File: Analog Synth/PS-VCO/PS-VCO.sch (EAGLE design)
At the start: 44 parts, among them IC1 TL084D, Q1 BC847BS, Q2 2N3906, Q3 2N3904, Q4 2N3904, Q5 2N7000

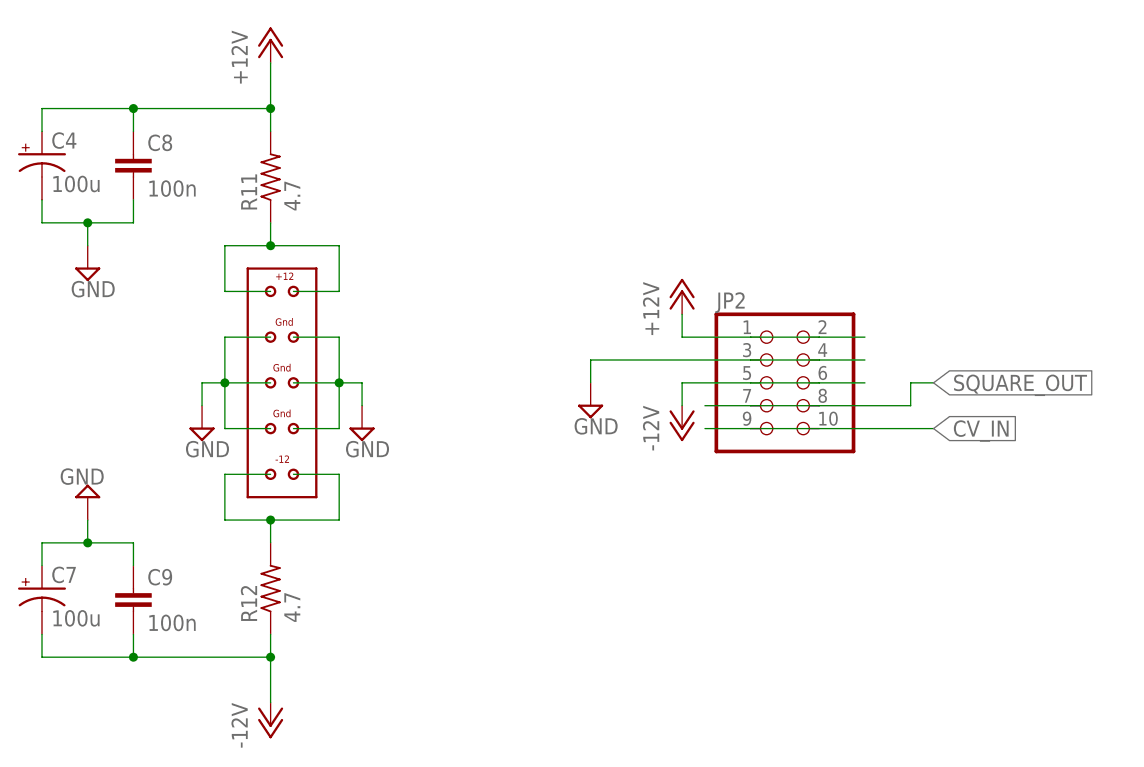
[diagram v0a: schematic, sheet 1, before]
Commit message: adding some data to the schematic
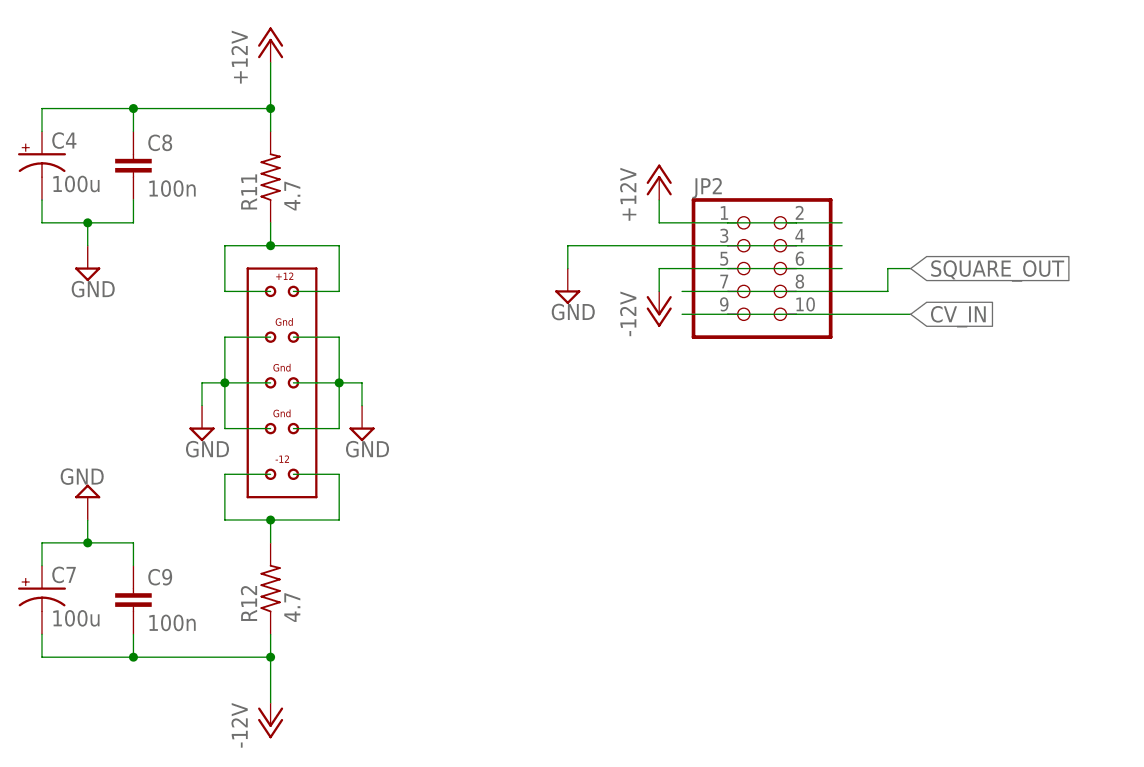
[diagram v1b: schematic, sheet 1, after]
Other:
- note added: "Experimental Data using +12 V and - 12 V supply rails output unloaded (disconnected) pot turned down to lowest frequency = 11 Hz +12 V line current draw = 8.6 mA -12 V line current draw = -8.6 mA 0 V frequency = 660 Hz +12 V line current draw = 10.1 mA -12 V line current draw = -10.0 mA pot turned up to highest frequency = 30 kHz +12 V line current draw = 14.1 mA -12 V line current draw = -13.7 mA"
- moved on the sheet: JP2
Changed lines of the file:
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@@
 <text x="-10.668" y="96.52" size="2.54" layer="98">2015-November</text>
 <text x="-36.83" y="78.74" size="2.54" layer="98">An attempt at creating a minimalistic VCO.</text>
+<text x="15.24" y="-10.16" size="1.778" layer="98">Experimental Data
+using +12 V and - 12 V supply rails
+output unloaded (disconnected)
+pot turned down to lowest frequency = 11 Hz
+  +12 V line current draw = 8.6 mA
+  -12 V line current draw = -8.6 mA
+0 V frequency = 660 Hz
+  +12 V line current draw = 10.1 mA
+  -12 V line current draw = -10.0 mA
+pot turned up to highest frequency = 30 kHz
+  +12 V line current draw = 14.1 mA
+  -12 V line current draw = -13.7 mA</text>
 </plain>
 <instances>
@@
 <instance part="R11" gate="G$1" x="-20.32" y="53.34" rot="R90"/>
 <instance part="R12" gate="G$1" x="-20.32" y="7.62" rot="R90"/>
-<instance part="JP2" gate="A" x="35.56" y="30.48"/>
+<instance part="JP2" gate="A" x="33.02" y="43.18"/>
 <instance part="C4" gate="G$1" x="-45.72" y="55.88"/>
 <instance part="C7" gate="G$1" x="-45.72" y="7.62"/>
@@
 <instance part="SUPPLY13" gate="GND" x="-40.64" y="43.18"/>
 <instance part="SUPPLY14" gate="GND" x="-40.64" y="17.78" rot="R180"/>
-<instance part="P+9" gate="1" x="25.4" y="40.64"/>
-<instance part="P-5" gate="1" x="25.4" y="25.4"/>
-<instance part="SUPPLY15" gate="GND" x="15.24" y="27.94"/>
+<instance part="P+9" gate="1" x="22.86" y="53.34"/>
+<instance part="P-5" gate="1" x="22.86" y="38.1"/>
+<instance part="SUPPLY15" gate="GND" x="12.7" y="40.64"/>
 </instances>
 <busses>
@@
 <segment>
 <pinref part="JP2" gate="A" pin="3"/>
-<wire x1="33.02" y1="33.02" x2="40.64" y2="33.02" width="0.1524" layer="91"/>
+<wire x1="30.48" y1="45.72" x2="38.1" y2="45.72" width="0.1524" layer="91"/>
 <pinref part="JP2" gate="A" pin="4"/>
-<wire x1="45.72" y1="33.02" x2="40.64" y2="33.02" width="0.1524" layer="91"/>
-<wire x1="33.02" y1="33.02" x2="15.24" y2="33.02" width="0.1524" layer="91"/>
+<wire x1="43.18" y1="45.72" x2="38.1" y2="45.72" width="0.1524" layer="91"/>
+<wire x1="30.48" y1="45.72" x2="12.7" y2="45.72" width="0.1524" layer="91"/>
 <pinref part="SUPPLY15" gate="GND" pin="GND"/>
-<wire x1="15.24" y1="33.02" x2="15.24" y2="30.48" width="0.1524" layer="91"/>
+<wire x1="12.7" y1="45.72" x2="12.7" y2="43.18" width="0.1524" layer="91"/>
 </segment>
 </net>
@@
 <pinref part="JP2" gate="A" pin="1"/>
 <pinref part="JP2" gate="A" pin="2"/>
-<wire x1="40.64" y1="35.56" x2="45.72" y2="35.56" width="0.1524" layer="91"/>
-<wire x1="40.64" y1="35.56" x2="33.02" y2="35.56" width="0.1524" layer="91"/>
-<wire x1="33.02" y1="35.56" x2="25.4" y2="35.56" width="0.1524" layer="91"/>
-<wire x1="25.4" y1="35.56" x2="25.4" y2="38.1" width="0.1524" layer="91"/>
+<wire x1="38.1" y1="48.26" x2="43.18" y2="48.26" width="0.1524" layer="91"/>
+<wire x1="38.1" y1="48.26" x2="30.48" y2="48.26" width="0.1524" layer="91"/>
+<wire x1="30.48" y1="48.26" x2="22.86" y2="48.26" width="0.1524" layer="91"/>
+<wire x1="22.86" y1="48.26" x2="22.86" y2="50.8" width="0.1524" layer="91"/>
 <pinref part="P+9" gate="1" pin="+12V"/>
 </segment>
@@
 <segment>
 <pinref part="JP2" gate="A" pin="5"/>
-<wire x1="33.02" y1="30.48" x2="40.64" y2="30.48" width="0.1524" layer="91"/>
+<wire x1="30.48" y1="43.18" x2="38.1" y2="43.18" width="0.1524" layer="91"/>
 <pinref part="JP2" gate="A" pin="6"/>
-<wire x1="45.72" y1="30.48" x2="40.64" y2="30.48" width="0.1524" layer="91"/>
-<wire x1="33.02" y1="30.48" x2="25.4" y2="30.48" width="0.1524" layer="91"/>
+<wire x1="43.18" y1="43.18" x2="38.1" y2="43.18" width="0.1524" layer="91"/>
+<wire x1="30.48" y1="43.18" x2="22.86" y2="43.18" width="0.1524" layer="91"/>
 <pinref part="P-5" gate="1" pin="-12V"/>
-<wire x1="25.4" y1="30.48" x2="25.4" y2="27.94" width="0.1524" layer="91"/>
+<wire x1="22.86" y1="43.18" x2="22.86" y2="40.64" width="0.1524" layer="91"/>
 </segment>
 </net>
@@
 <segment>
 <pinref part="JP2" gate="A" pin="7"/>
-<wire x1="33.02" y1="27.94" x2="27.94" y2="27.94" width="0.1524" layer="91"/>
-<wire x1="33.02" y1="27.94" x2="40.64" y2="27.94" width="0.1524" layer="91"/>
+<wire x1="30.48" y1="40.64" x2="25.4" y2="40.64" width="0.1524" layer="91"/>
+<wire x1="30.48" y1="40.64" x2="38.1" y2="40.64" width="0.1524" layer="91"/>
 <pinref part="JP2" gate="A" pin="8"/>
-<wire x1="53.34" y1="30.48" x2="50.8" y2="30.48" width="0.1524" layer="91"/>
-<wire x1="50.8" y1="30.48" x2="50.8" y2="27.94" width="0.1524" layer="91"/>
-<wire x1="50.8" y1="27.94" x2="40.64" y2="27.94" width="0.1524" layer="91"/>
-<label x="53.34" y="30.48" size="1.778" layer="95" xref="yes"/>
+<wire x1="50.8" y1="43.18" x2="48.26" y2="43.18" width="0.1524" layer="91"/>
+<wire x1="48.26" y1="43.18" x2="48.26" y2="40.64" width="0.1524" layer="91"/>
+<wire x1="48.26" y1="40.64" x2="38.1" y2="40.64" width="0.1524" layer="91"/>
+<label x="50.8" y="43.18" size="1.778" layer="95" xref="yes"/>
 </segment>
 </net>
@@
 <segment>
 <pinref part="JP2" gate="A" pin="9"/>
-<wire x1="33.02" y1="25.4" x2="27.94" y2="25.4" width="0.1524" layer="91"/>
-<wire x1="33.02" y1="25.4" x2="40.64" y2="25.4" width="0.1524" layer="91"/>
+<wire x1="30.48" y1="38.1" x2="25.4" y2="38.1" width="0.1524" layer="91"/>
+<wire x1="30.48" y1="38.1" x2="38.1" y2="38.1" width="0.1524" layer="91"/>
 <pinref part="JP2" gate="A" pin="10"/>
-<label x="53.34" y="25.4" size="1.778" layer="95" xref="yes"/>
-<wire x1="40.64" y1="25.4" x2="53.34" y2="25.4" width="0.1524" layer="91"/>
-</segment>
-</net>
+<label x="50.8" y="38.1" size="1.778" layer="95" xref="yes"/>
+<wire x1="38.1" y1="38.1" x2="50.8" y2="38.1" width="0.1524" layer="91"/>
+</segment>
+</net>
